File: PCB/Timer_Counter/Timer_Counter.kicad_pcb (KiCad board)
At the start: 2 copper layers, 5 parts, among them J1 Conn_01x20, J2 Conn_01x20, J4 Conn_01x03

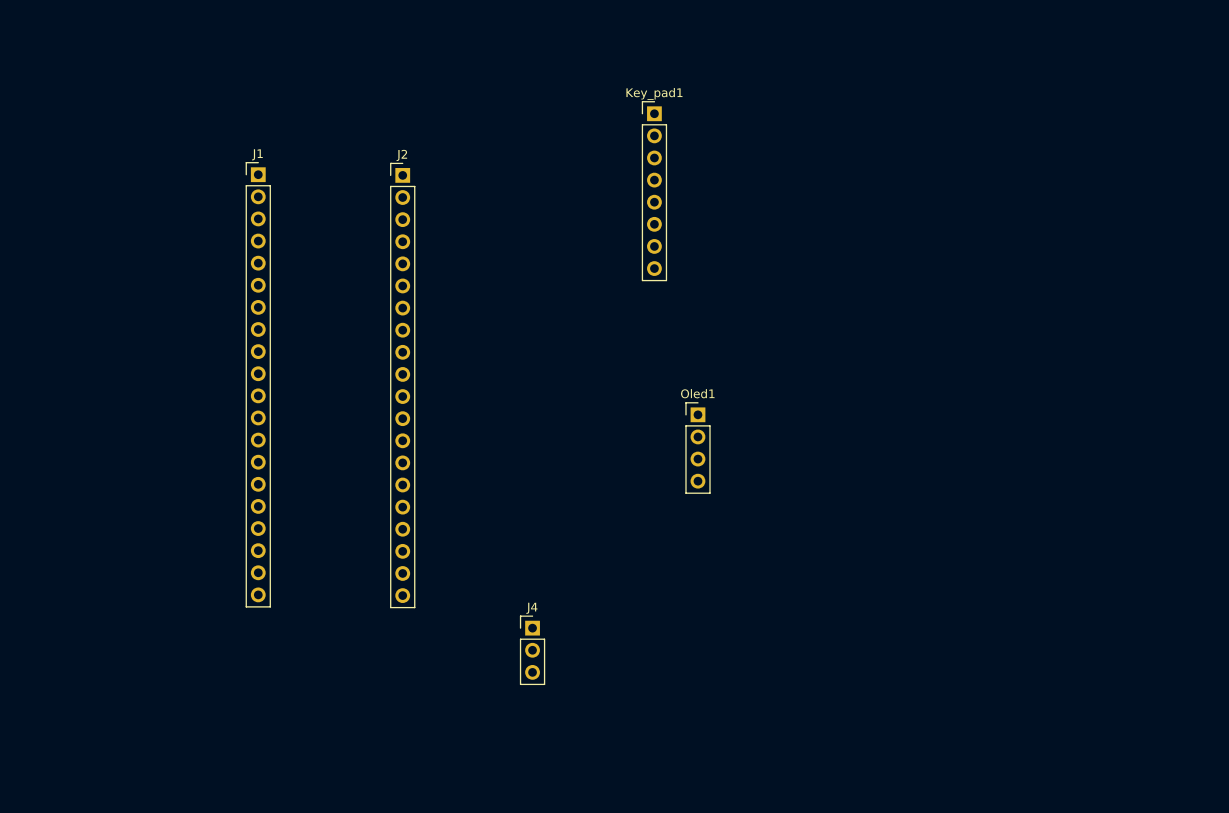
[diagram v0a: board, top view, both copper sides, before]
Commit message: Them pcb mơi sửa vào
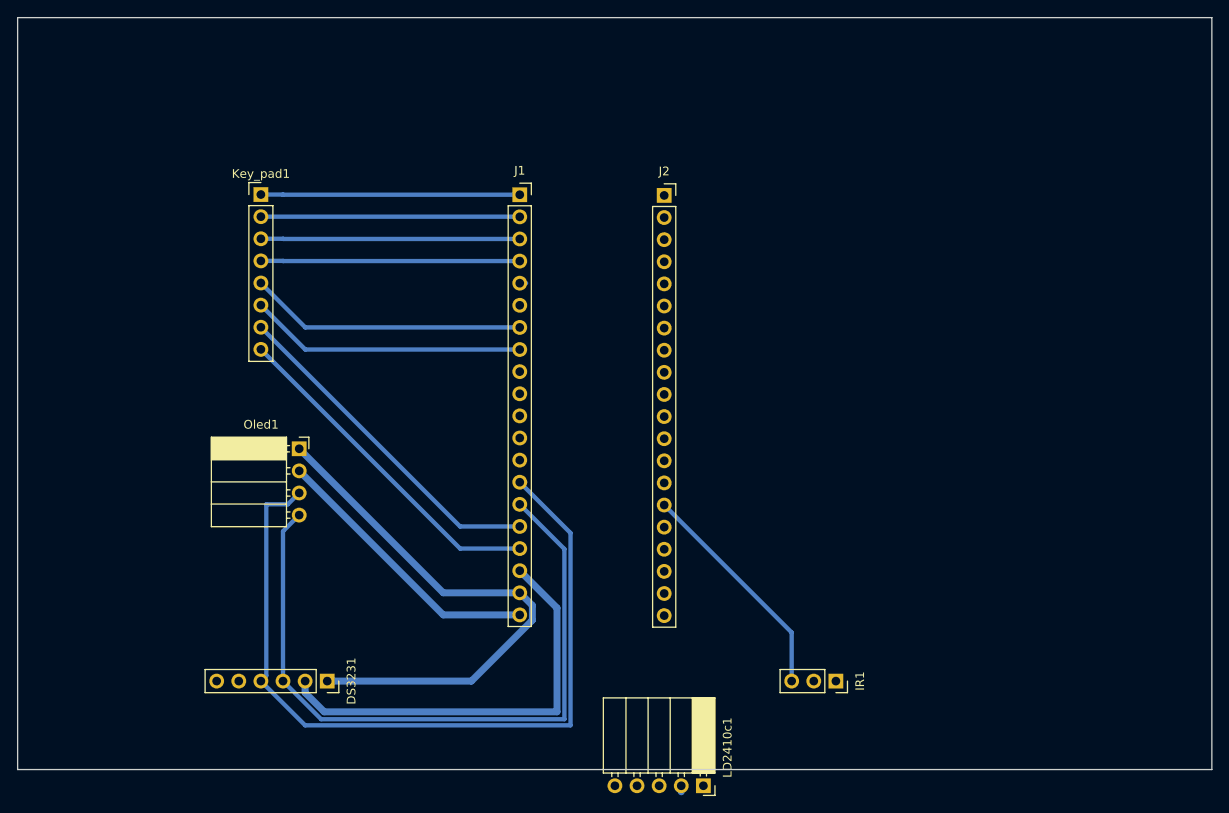
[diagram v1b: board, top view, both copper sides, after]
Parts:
- added DS3231: Conn_01x06, Connector_PinSocket_2.54mm:PinSocket_1x06_P2.54mm_Vertical, F.Cu at (121.9, 127.0)
- added LD2410c1: Conn_01x05, Connector_PinSocket_2.54mm:PinSocket_1x05_P2.54mm_Horizontal, F.Cu at (165.1, 139.0)
- IR1: renamed from J4; footprint Connector_PinHeader_2.54mm:PinHeader_1x03_P2.54mm_Vertical -> Connector_PinSocket_2.54mm:PinSocket_1x03_P2.54mm_Vertical
- J1, J2: footprint Connector_PinHeader_2.54mm:PinHeader_1x20_P2.54mm_Vertical -> Connector_PinSocket_2.54mm:PinSocket_1x20_P2.54mm_Vertical
- Oled1: footprint Connector_PinHeader_2.54mm:PinHeader_1x04_P2.54mm_Vertical -> Connector_PinSocket_2.54mm:PinSocket_1x04_P2.54mm_Horizontal
- moved Key_pad1 46.1 mm to (114.3, 71.1)
- moved Oled1 46.0 mm to (118.7, 100.3)
- moved IR1 35.4 mm to (180.3, 127.0), turned to -90 degrees
- moved J1 30.1 mm to (144.0, 71.1)
- moved J2 30.1 mm to (160.6, 71.2)
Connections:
- J1 pad 1: unconnected-(J1-Pin_1-Pad1) -> /B12
- J1 pad 14: unconnected-(J1-Pin_14-Pad14) -> /SCL
- J1 pad 15: unconnected-(J1-Pin_15-Pad15) -> /SDA
- J1 pad 16: unconnected-(J1-Pin_16-Pad16) -> /B08
- J1 pad 17: unconnected-(J1-Pin_17-Pad17) -> /B09
- J1 pad 18: unconnected-(J1-Pin_18-Pad18) -> +5V
- J1 pad 19: unconnected-(J1-Pin_19-Pad19) -> GND
- J1 pad 2: unconnected-(J1-Pin_2-Pad2) -> /B13
- J1 pad 20: unconnected-(J1-Pin_20-Pad20) -> +3.3V
- J1 pad 3: unconnected-(J1-Pin_3-Pad3) -> /B14
- J1 pad 4: unconnected-(J1-Pin_4-Pad4) -> /B15
- J1 pad 5: unconnected-(J1-Pin_5-Pad5) -> /OUT
- J1 pad 7: unconnected-(J1-Pin_7-Pad7) -> /A10
- J1 pad 8: unconnected-(J1-Pin_8-Pad8) -> /A11
- J2 pad 15: unconnected-(J2-Pin_15-Pad15) -> /A1
- Key_pad1 pad 1: /B13 -> /B12
- Key_pad1 pad 2: /B12 -> /B13
- Key_pad1 pad 3: /B15 -> /B14
- Key_pad1 pad 4: /B14 -> /B15
- Key_pad1 pad 5: /A11 -> /A10
- Key_pad1 pad 6: /A10 -> /A11
- Key_pad1 pad 8: /B07 -> /B09
- Oled1 pad 2: +5V -> +3.3V
- Oled1 pad 3: /<NO NET> -> /SCL
- Oled1 pad 4: /B11 -> /SDA
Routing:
- net /SCL: track 0.00 -> 93.5 mm
- net /SDA: track 0.00 -> 80.8 mm
- net GND: track 0.00 -> 63.1 mm
- net +5V: track 0.00 -> 49.2 mm
- net /B09: track 0.00 -> 39.2 mm
- net /B08: track 0.00 -> 39.2 mm
- net +3.3V: track 0.00 -> 32.2 mm
- net /A11: track 0.00 -> 31.8 mm
- net /A10: track 0.00 -> 31.8 mm
- net /B15: track 0.00 -> 29.7 mm
- net /B13: track 0.00 -> 29.7 mm
- net /B14: track 0.00 -> 29.7 mm
- net /B12: track 0.00 -> 29.7 mm
- net /A1: track 0.00 -> 26.3 mm
- net /OUT: track 0.00 -> 0.73 mm
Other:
- board outline added: 137.2 x 86.4 mm
